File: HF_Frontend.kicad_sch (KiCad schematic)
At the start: 7 parts

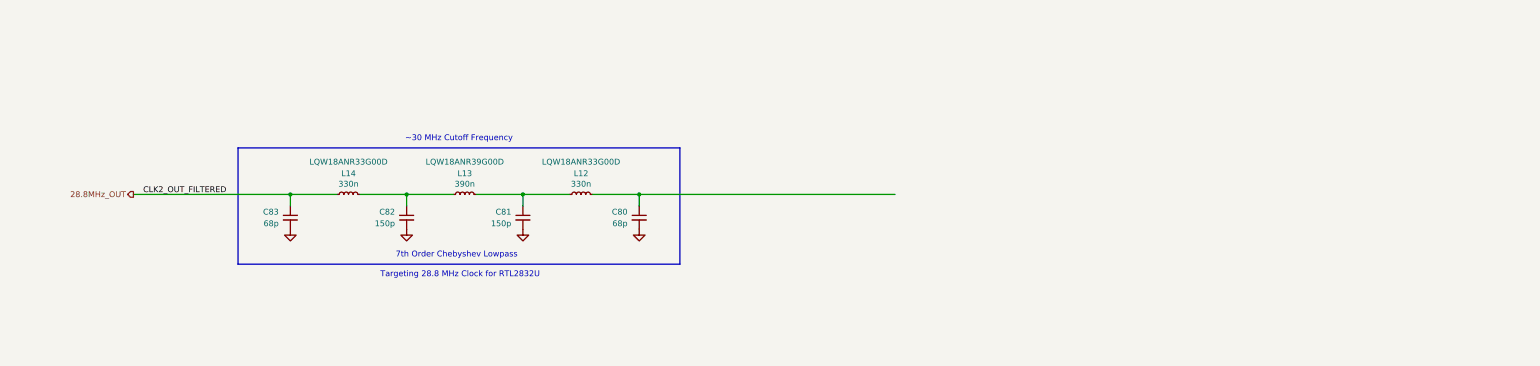
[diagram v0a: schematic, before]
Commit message: Schematic progress
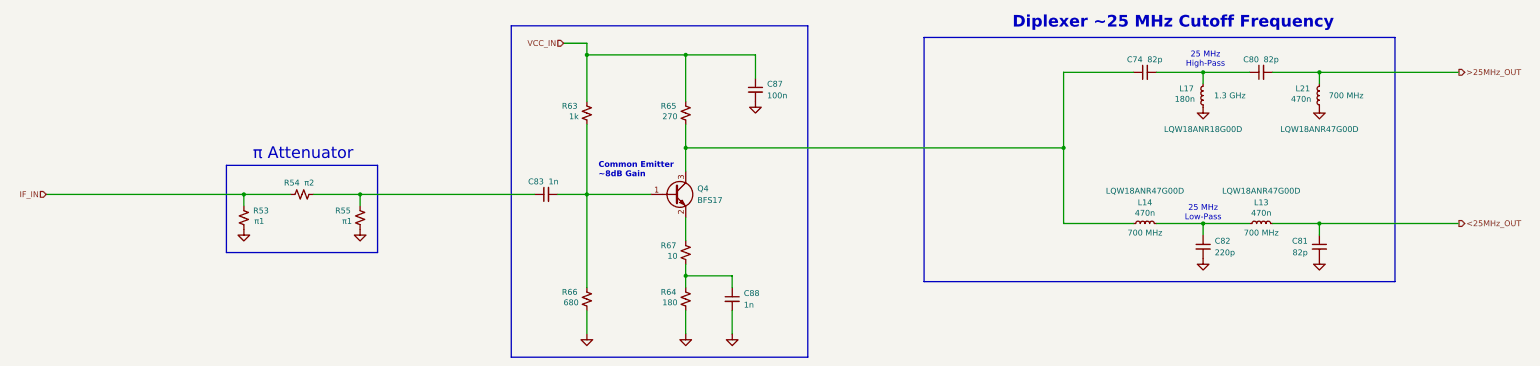
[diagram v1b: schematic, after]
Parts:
- removed L12: 330n, libraries:Worthington_L_0603, symbol Device:L_Small
- added C74: 82p, libraries:Worthington_C_0402, symbol Device:C_Small
- added C87: 100n, libraries:Worthington_C_0402, symbol Device:C_Small
- added C88: 1n, libraries:Worthington_C_0402, symbol Device:C_Small
- added L17: 180n, libraries:Worthington_L_0603, symbol Device:L_Small
- added L21: 470n, libraries:Worthington_L_0603, symbol Device:L_Small
- added Q4: BFS17, symbol Device:Q_NPN
- added R53, R55: π1, libraries:Worthington_R_0402, symbol Device:R_Small_US
- added R54: π2, libraries:Worthington_R_0402, symbol Device:R_Small_US
- added R63: 1k, libraries:Worthington_R_0402, symbol Device:R_Small_US
- added R64: 180, libraries:Worthington_R_0402, symbol Device:R_Small_US
- added R65: 270, libraries:Worthington_R_0402, symbol Device:R_Small_US
- added R66: 680, libraries:Worthington_R_0402, symbol Device:R_Small_US
- added R67: 10, libraries:Worthington_R_0402, symbol Device:R_Small_US
- C80: value 68p -> 82p; footprint Capacitor_SMD:C_0603_1608Metric_Pad1.08x0.95mm_HandSolder -> libraries:Worthington_C_0402
- C81: value 150p -> 82p
- C82: value 150p -> 220p
- C83: value 68p -> 1n; footprint Capacitor_SMD:C_0603_1608Metric_Pad1.08x0.95mm_HandSolder -> libraries:Worthington_C_0402
- L13: value 390n -> 470n; Murata LQW18ANR39G00D -> LQW18ANR47G00D; Self-Resonance (none) -> 700 MHz
- L14: value 330n -> 470n; Murata LQW18ANR33G00D -> LQW18ANR47G00D; Self-Resonance (none) -> 700 MHz
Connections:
- net GND: now also C87.2, C88.2, L17.1, L21.1, R53.1, R55.1, R64.1, R66.1; no longer C80.2, C83.2
- net at C80.1: now also C74.2, L17.2
- net <25MHz_OUT: now reaches C81.1, L13.2
- net 28.8MHz_OUT: no longer names the net of C83.1
- net 28.8MHz_OUT: now also R54.2, R55.2; no longer L14.1
- new net: C83.2, Q4.1 (B), R63.1, R66.2
- new net: Q4.2 (E), R67.2
- new net: C74.1, L14.1, Q4.3 (C), R65.1
- new net: C88.1, R64.2, R67.1
- new net >25MHz_OUT: C80.2, L21.2
- new net IF_IN: R53.2, R54.1
- new net VCC_IN: C87.1, R63.2, R65.2
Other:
- note added: "25 MHz High-Pass"
- note added: "25 MHz Low-Pass"
- note added: "Common Emitter ~8dB Gain"
- note added: "Diplexer ~25 MHz Cutoff Frequency"
- note added: "π Attenuator"
- note removed: "7th Order Chebyshev Lowpass"
- note removed: "Targeting 28.8 MHz Clock for RTL2832U"
- note removed: "~30 MHz Cutoff Frequency"
- moved on the sheet: C81, C82, L13, L14
